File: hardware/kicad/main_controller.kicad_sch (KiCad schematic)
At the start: 24 parts, among them J3 JTAG_10PIN, SW1 RESET, SW2 BOOT, U6 ESP32-S3-MINI-1, Y1 32.768 kHz

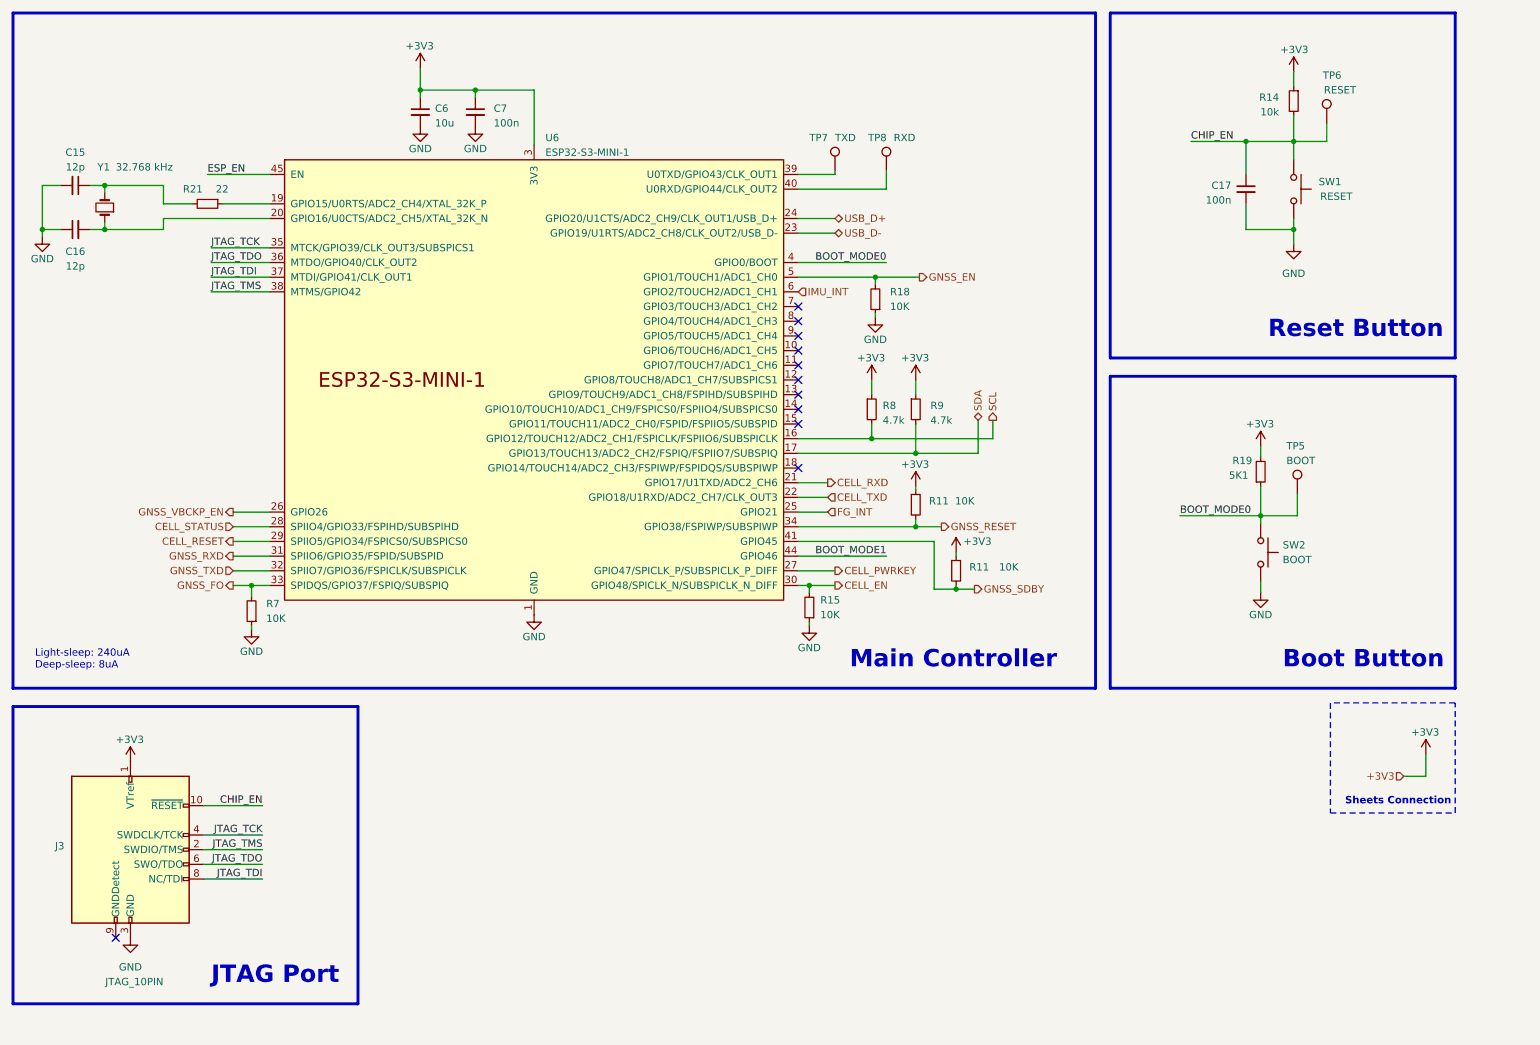
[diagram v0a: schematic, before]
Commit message: wip: revision 2
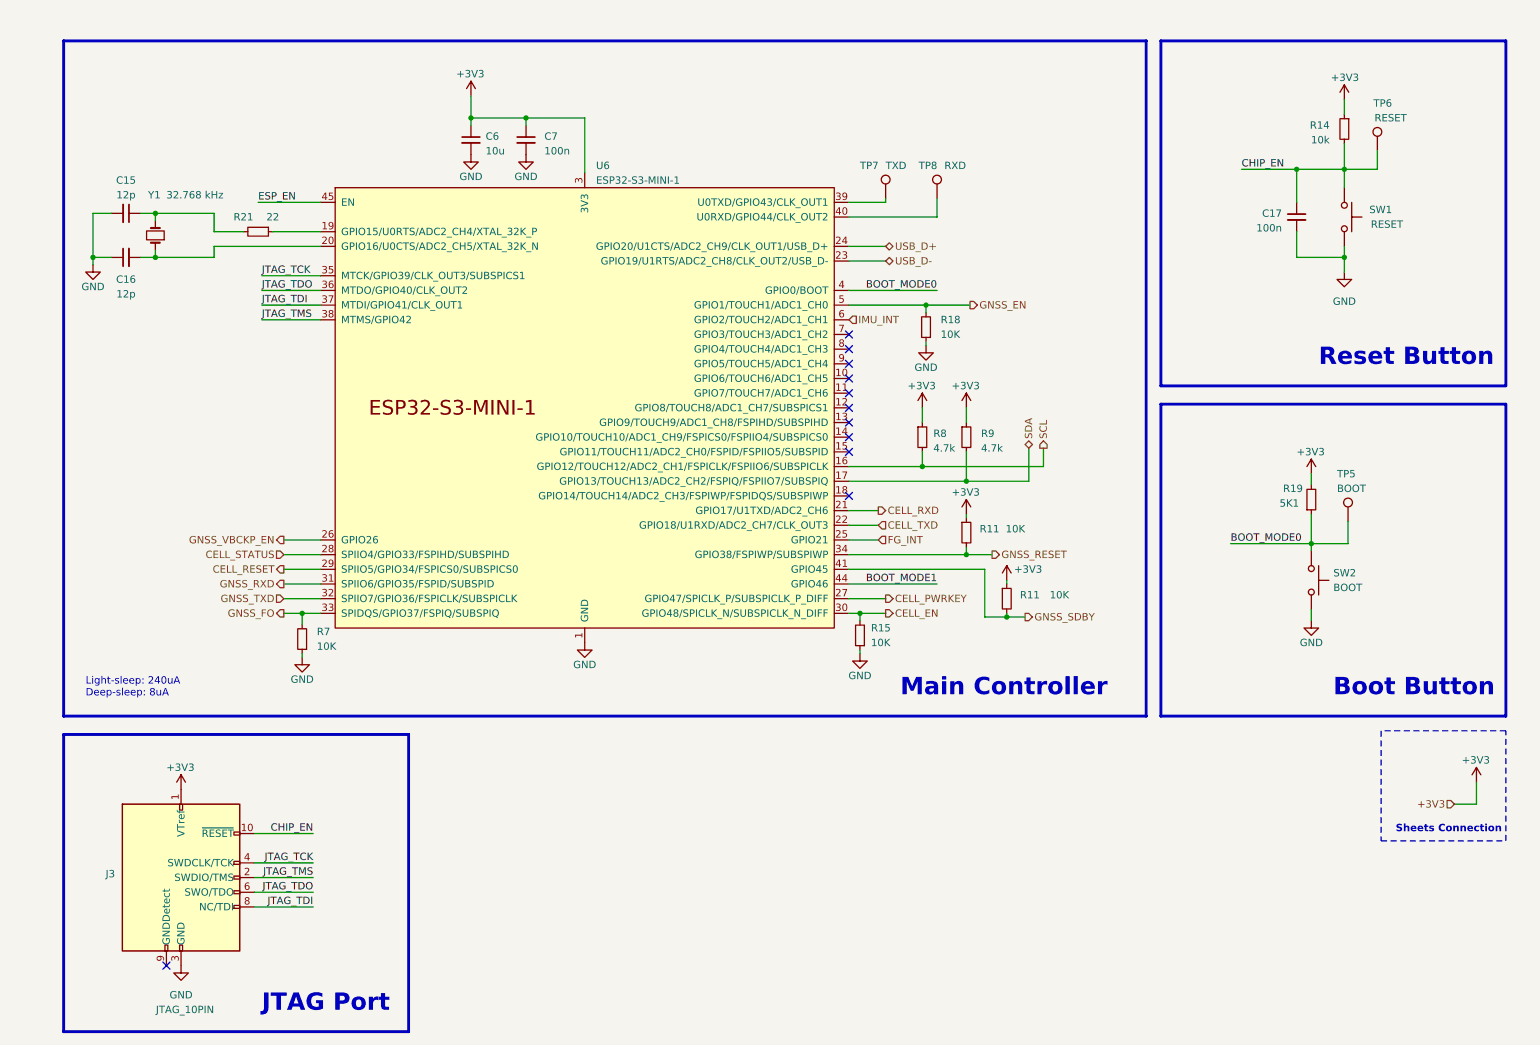
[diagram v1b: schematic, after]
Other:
- moved on the sheet: C15, C16, C17, C6, C7, J3, R11, R14, R15, R18, R19, R21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
